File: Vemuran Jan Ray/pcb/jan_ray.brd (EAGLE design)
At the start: 58.9 x 67.3 mm, 38 parts, among them IC1 LM4558, X1 2510-

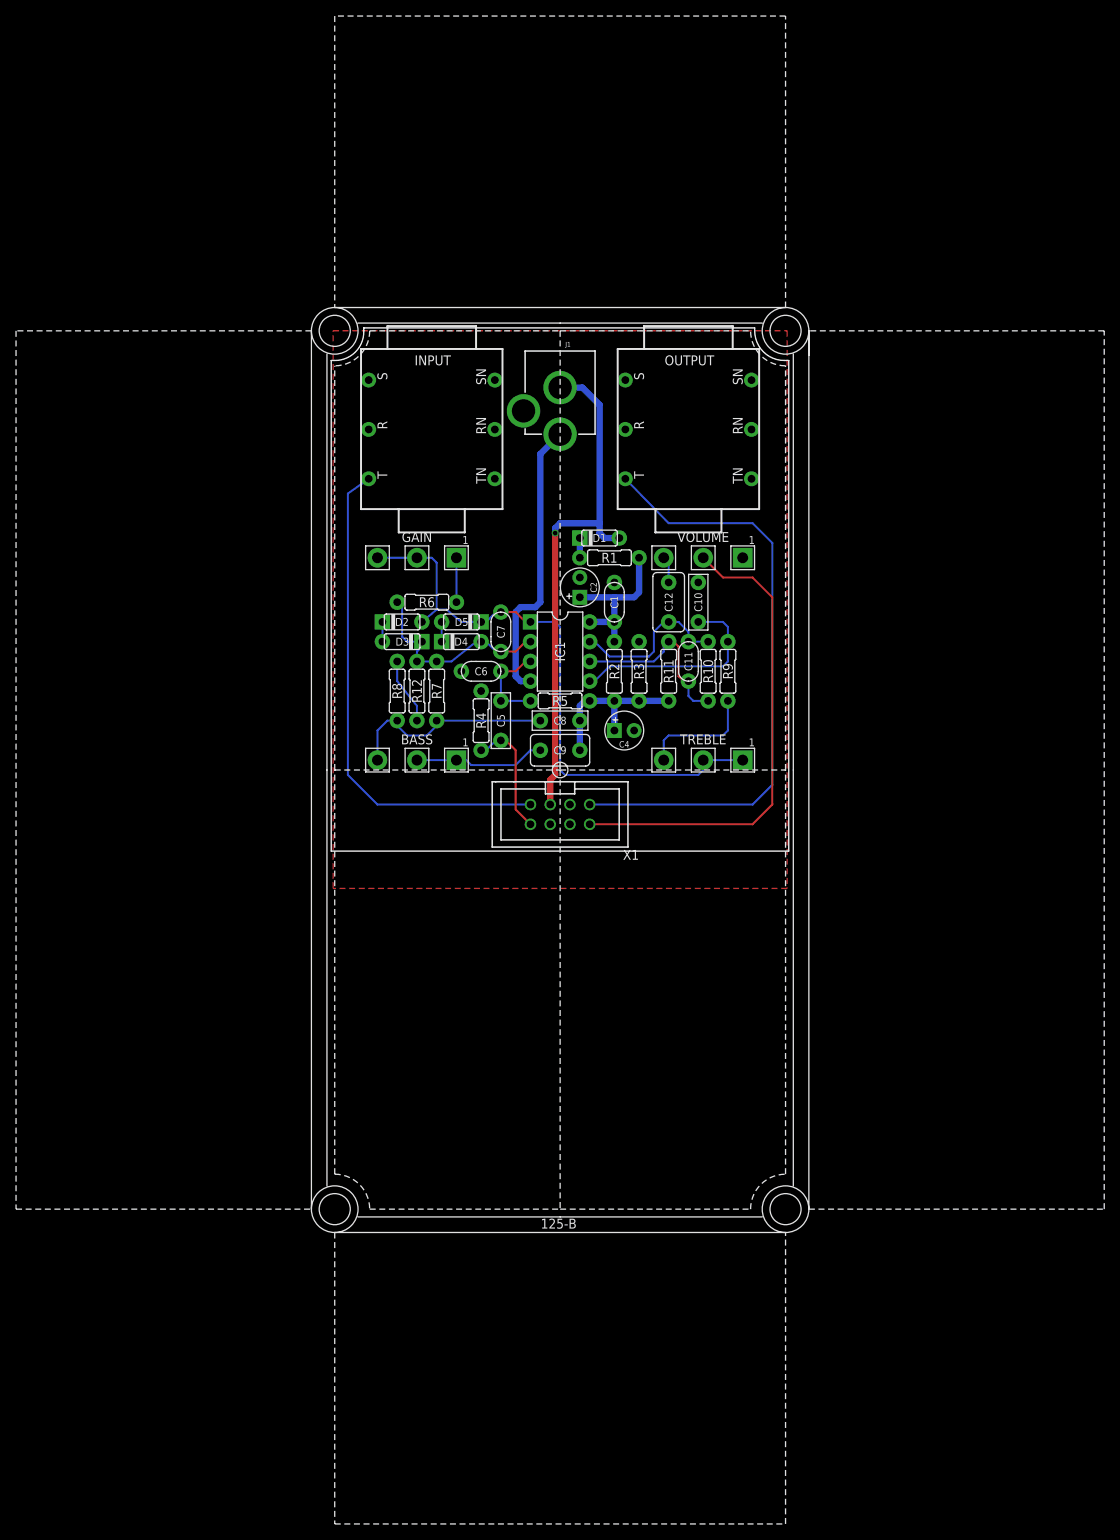
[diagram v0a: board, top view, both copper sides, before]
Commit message: 20170712
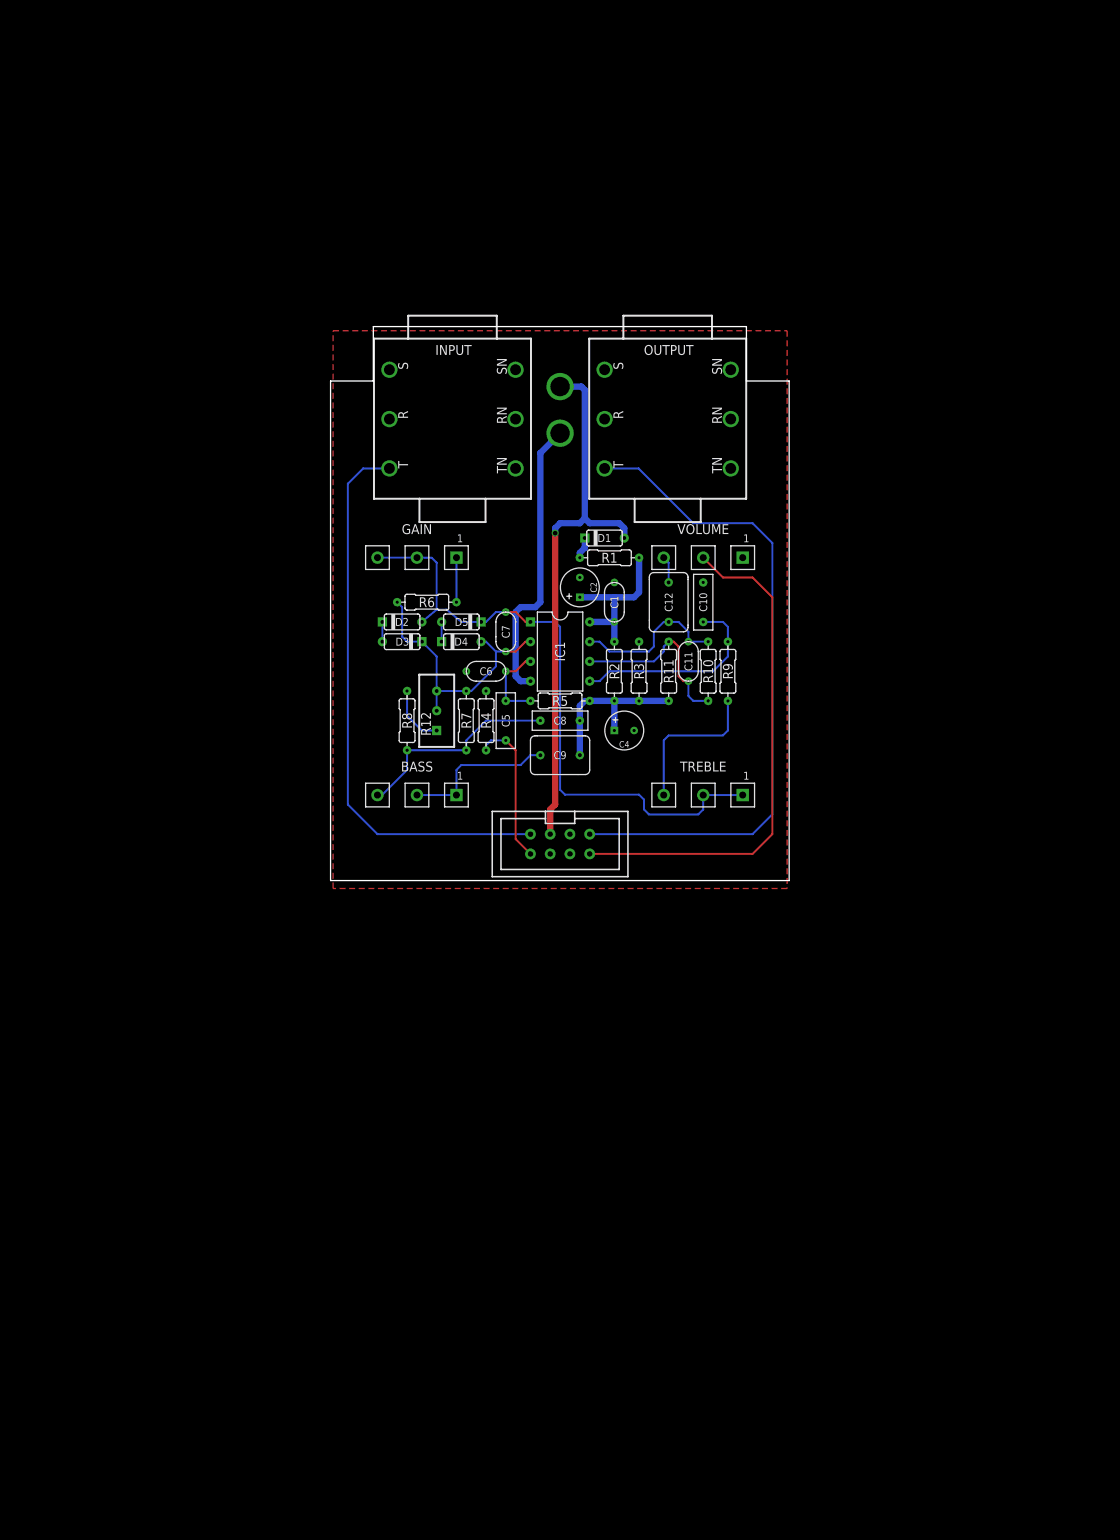
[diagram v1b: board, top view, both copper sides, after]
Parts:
- C12, C9: device pedals-capacitors-film:BOX_MED -> pedals-capacitors-film:BOX_BIG
- J1: value (none) -> POWER_JACK
- R12: value 3.9k -> (none); device pedals-resistors:R0207/3 -> pedals-potentiometers:RTRIM3296W
- U$1: device pedals-enclosures:125B -> pedals-pcb:125B_PCB
- moved U$1 32.2 mm to (-0.32, 2.92)
- moved R7 5.39 mm to (17.1, 22.2)
- moved R8 4.02 mm to (9.53, 22.2)
- moved X1 3.81 mm to (29.2, 6.35)
- moved R12 3.59 mm to (13.3, 23.5), turned to 0 degrees
- moved BASS 3.49 mm to (10.8, 13.7)
- moved TREBLE 3.49 mm to (47.6, 13.7)
- moved INPUT 2.98 mm to (15.4, 61.0)
- moved OUTPUT 2.98 mm to (43.1, 61.0)
- moved GAIN 1.02 mm to (10.8, 44.2)
- moved VOLUME 1.02 mm to (47.6, 44.2)
- moved C5 0.64 mm to (22.2, 22.2)
- moved C7 0.64 mm to (22.2, 33.7)
- moved C10 0.63 mm to (47.6, 37.5)
- moved C6 0.63 mm to (19.7, 28.6)
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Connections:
- net N$5: now also R12.3
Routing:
- net N$5: track 26.9 -> 35.4 mm
- net N$2: track 64.6 -> 72.5 mm
- net N$4: track 78.0 -> 85.0 mm
- net N$6: track 77.9 -> 82.8 mm
- net N$12: track 15.1 -> 19.6 mm
- net OUT: track 62.2 -> 66.0 mm
- net +9V: track 67.1 -> 70.7 mm
- net IN: track 15.8 -> 19.4 mm
- net N$13: track 16.9 -> 19.9 mm
- net N$3: track 12.0 -> 10.7 mm
- net N$14: track 27.4 -> 26.3 mm
- net N$16: track 21.2 -> 20.3 mm
- net N$10: track 8.51 -> 7.77 mm
- net VB: track 21.2 -> 21.9 mm
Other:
- board size 58.9 x 67.3 mm -> 59 x 71.3 mm
